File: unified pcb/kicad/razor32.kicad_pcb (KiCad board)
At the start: 4 copper layers, 138 x 57 mm, 33 parts

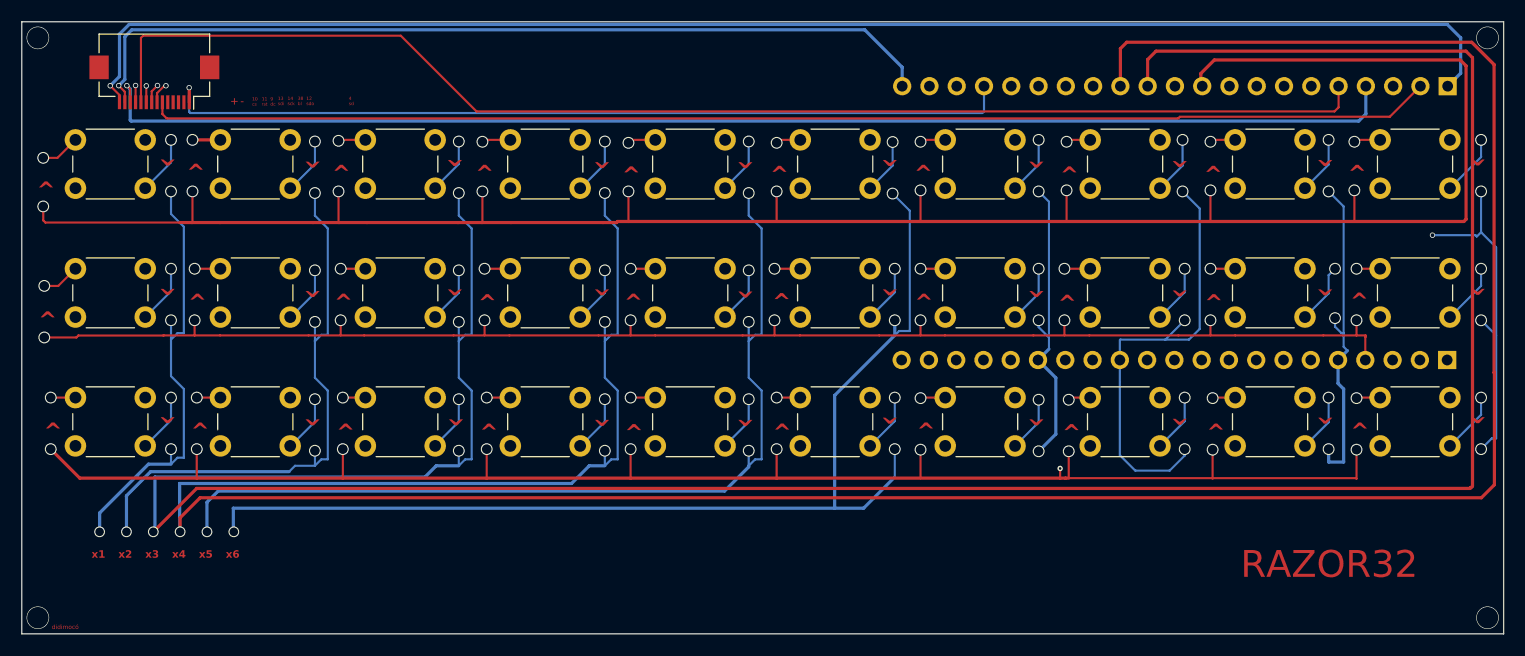
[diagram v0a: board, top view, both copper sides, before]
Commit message: Clean PCB
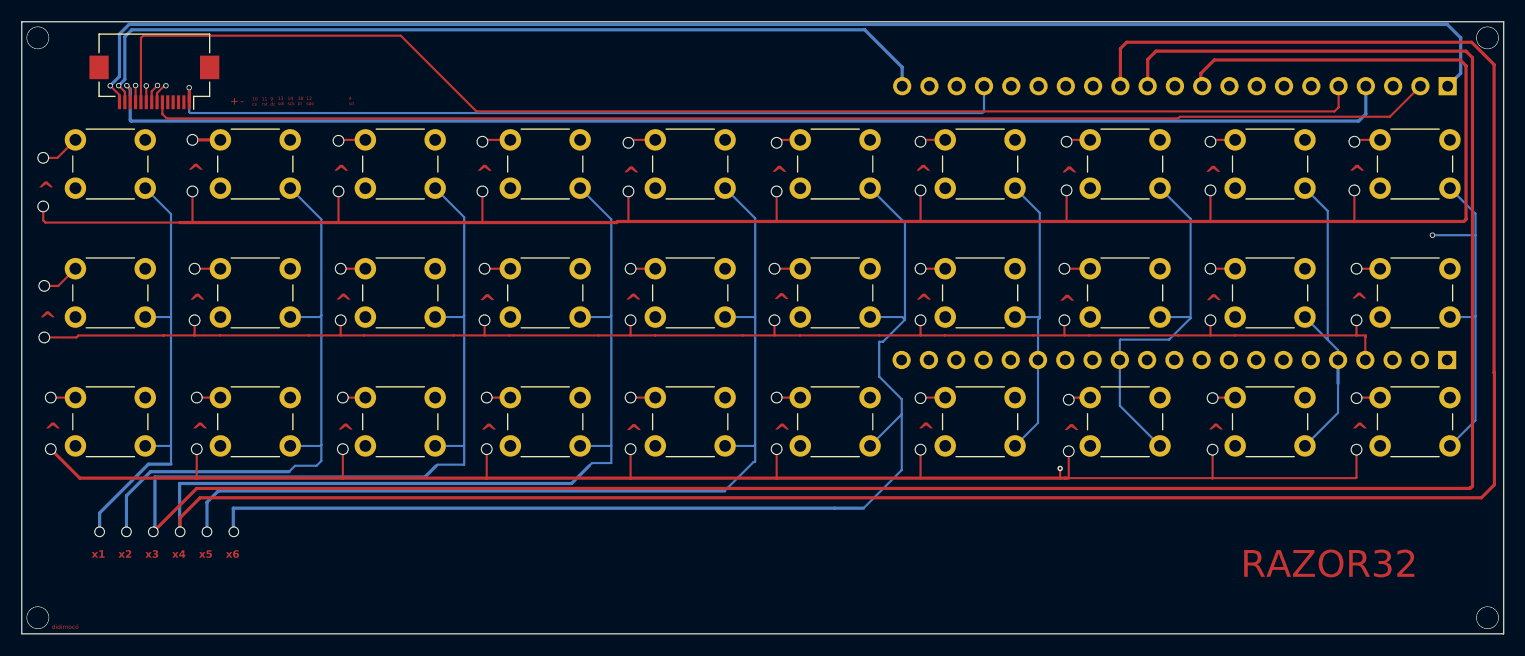
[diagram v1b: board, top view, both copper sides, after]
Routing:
- net x8: track 58.7 -> 35.0 mm, vias 6 -> 0
- net x9: track 47.4 -> 29.6 mm, vias 6 -> 0
- net x10: track 96.5 -> 79.6 mm, vias 7 -> 1
- net x1: track 223.7 -> 207.4 mm, vias 7 -> 1
- net x7: track 44.4 -> 28.2 mm, vias 6 -> 0
- net x6: track 311.7 -> 296.3 mm, vias 7 -> 1
- net x3: track 279.5 -> 264.6 mm, vias 7 -> 1
- net x5: track 269.3 -> 254.6 mm, vias 7 -> 1
- net x2: track 230.0 -> 215.5 mm, vias 7 -> 1
- net x4: track 296.1 -> 281.7 mm, vias 7 -> 1
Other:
- board text removed: "42"
- board text removed: "47"
